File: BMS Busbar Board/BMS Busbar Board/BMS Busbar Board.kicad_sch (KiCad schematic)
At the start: 17 parts, among them J1 Conn_01x05_MountingPin, J2 Conn_01x05_MountingPin

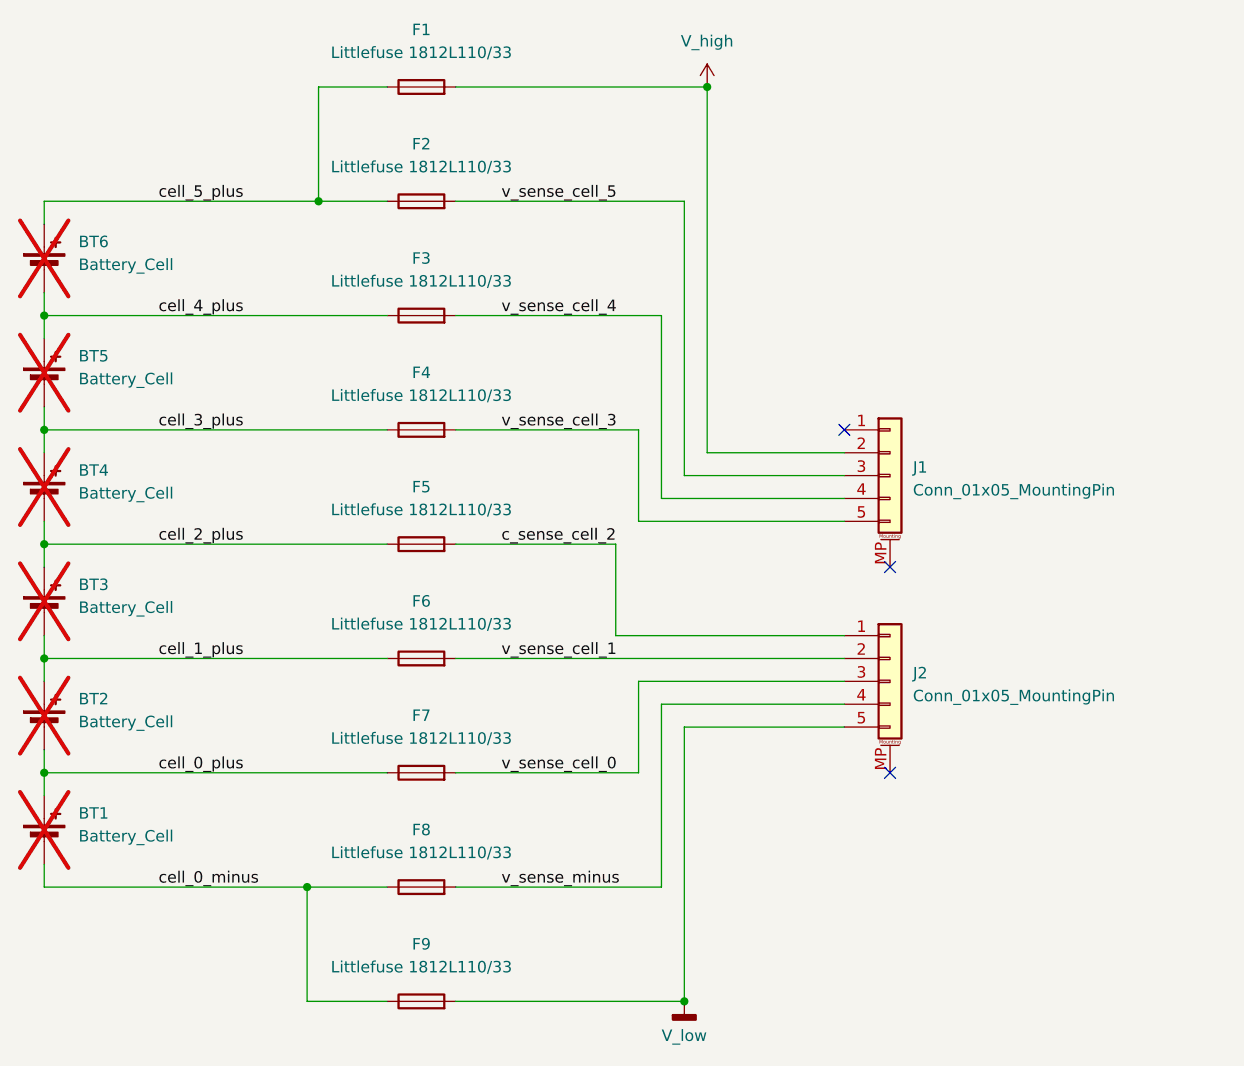
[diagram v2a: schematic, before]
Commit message: new connector added
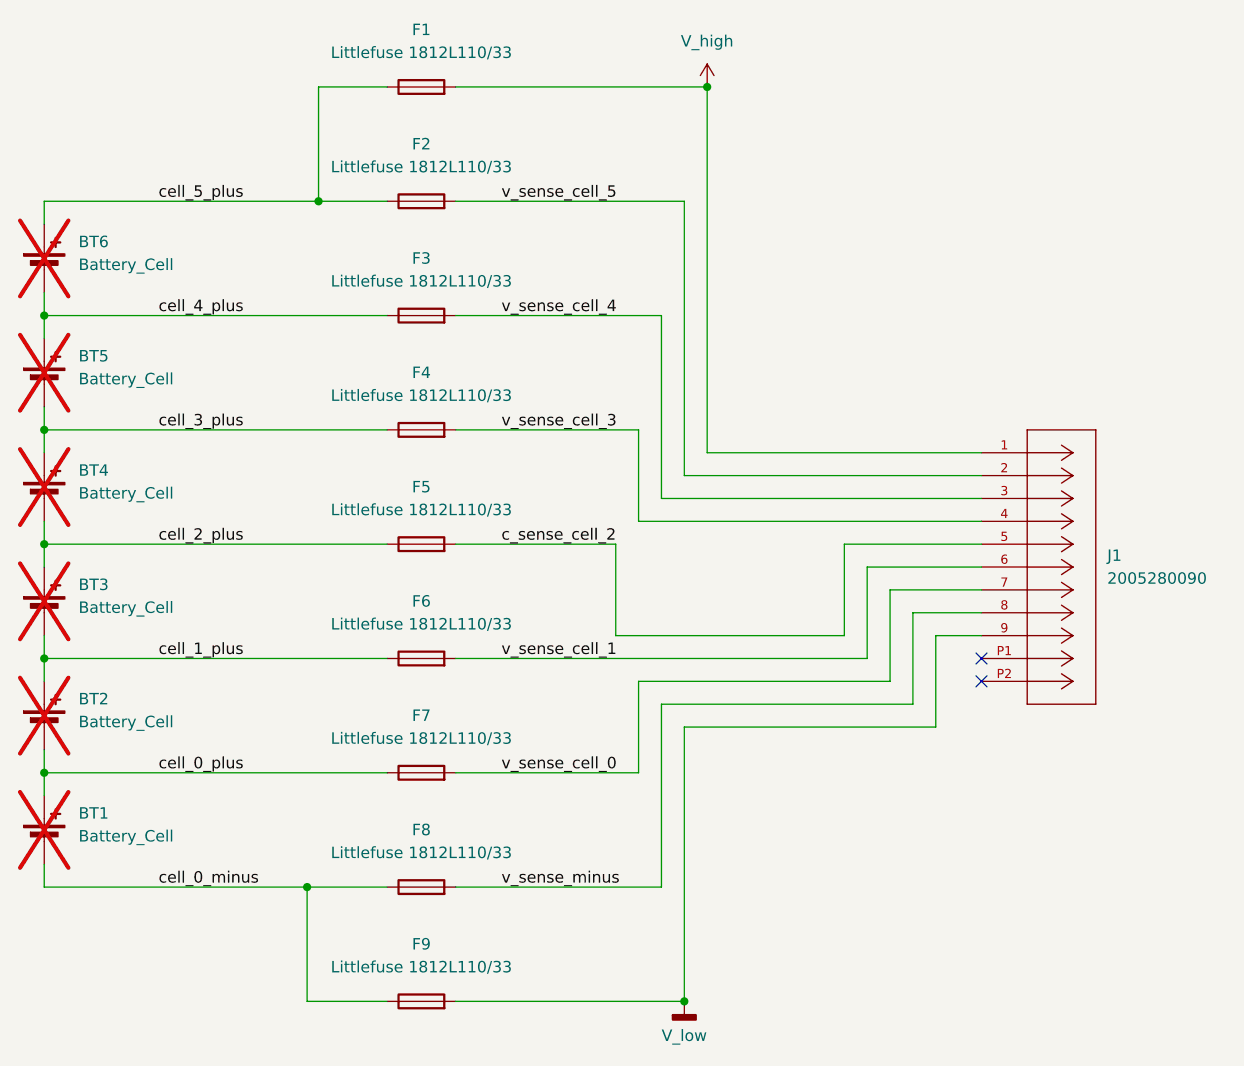
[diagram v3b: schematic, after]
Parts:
- removed J1, J2: Conn_01x05_MountingPin, FS_4_Global_Footprint_Library:512810598, symbol Connector_Generic_MountingPin:Conn_01x05_MountingPin
- added J1: 2005280090, FS_4_Global_Footprint_Library:CON_2005280090_MOL, symbol FS_4_Global_Symbol_Library:2005280090
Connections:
- net V_high: now also J1.1
- net V_low: now also J1.9
- net c_sense_cell_2: now also J1.5
- net v_sense_cell_0: now also J1.7
- net v_sense_cell_1: now also J1.6
- net v_sense_cell_3: now also J1.4
- net v_sense_cell_4: now also J1.3
- net v_sense_cell_5: now also J1.2
- net v_sense_minus: now also J1.8
- no-connect marks 3 -> 2
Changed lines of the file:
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@@
 	)
 	(no_connect
-		(at 157.48 104.14)
+		(at 167.64 93.98)
 	)
 	(no_connect
-		(at 157.48 81.28)
-	)
-	(no_connect
-		(at 152.4 66.04)
-	)
-	(wire
-		(pts
-			(xy 137.16 68.58) (xy 152.4 68.58)
+		(at 167.64 91.44)
+	)
+	(wire
+		(pts
+			(xy 160.02 86.36) (xy 167.64 86.36)
+		)
+		(stroke
+			(width 0)
+			(type default)
+		)
+	)
+	(wire
+		(pts
+			(xy 137.16 68.58) (xy 167.64 68.58)
 		)
 		(stroke
@@
 	(wire
 		(pts
-			(xy 134.62 99.06) (xy 152.4 99.06)
+			(xy 134.62 99.06) (xy 162.56 99.06)
 		)
 		(stroke
@@
 	(wire
 		(pts
-			(xy 129.54 93.98) (xy 152.4 93.98)
+			(xy 129.54 93.98) (xy 157.48 93.98)
 		)
 		(stroke
@@
 	(wire
 		(pts
-			(xy 109.22 91.44) (xy 152.4 91.44)
+			(xy 109.22 91.44) (xy 154.94 91.44)
 		)
 		(stroke
@@
 	(wire
 		(pts
+			(xy 157.48 93.98) (xy 157.48 83.82)
+		)
+		(stroke
+			(width 0)
+			(type default)
+		)
+	)
+	(wire
+		(pts
 			(xy 101.6 91.44) (xy 63.5 91.44)
 		)
@@
 	(wire
 		(pts
+			(xy 162.56 99.06) (xy 162.56 88.9)
+		)
+		(stroke
+			(width 0)
+			(type default)
+		)
+	)
+	(wire
+		(pts
 			(xy 63.5 114.3) (xy 63.5 116.84)
 		)
@@
 	(wire
 		(pts
+			(xy 154.94 91.44) (xy 154.94 81.28)
+		)
+		(stroke
+			(width 0)
+			(type default)
+		)
+	)
+	(wire
+		(pts
 			(xy 63.5 88.9) (xy 63.5 91.44)
 		)
@@
 	(wire
 		(pts
+			(xy 152.4 88.9) (xy 152.4 78.74)
+		)
+		(stroke
+			(width 0)
+			(type default)
+		)
+	)
+	(wire
+		(pts
 			(xy 63.5 104.14) (xy 63.5 106.68)
 		)
@@
 	(wire
 		(pts
-			(xy 129.54 76.2) (xy 152.4 76.2)
+			(xy 162.56 88.9) (xy 167.64 88.9)
+		)
+		(stroke
+			(width 0)
+			(type default)
+		)
+	)
+	(wire
+		(pts
+			(xy 129.54 76.2) (xy 167.64 76.2)
 		)
 		(stroke
@@
 	(wire
 		(pts
+			(xy 160.02 96.52) (xy 160.02 86.36)
+		)
+		(stroke
+			(width 0)
+			(type default)
+		)
+	)
+	(wire
+		(pts
 			(xy 132.08 53.34) (xy 132.08 73.66)
 		)
@@
 	(wire
 		(pts
-			(xy 132.08 96.52) (xy 152.4 96.52)
-		)
-		(stroke
-			(width 0)
-			(type default)
-		)
-	)
-	(wire
-		(pts
-			(xy 132.08 73.66) (xy 152.4 73.66)
+			(xy 132.08 96.52) (xy 160.02 96.52)
+		)
+		(stroke
+			(width 0)
+			(type default)
+		)
+	)
+	(wire
+		(pts
+			(xy 132.08 73.66) (xy 167.64 73.66)
 		)
 		(stroke
@@
 	(wire
 		(pts
-			(xy 134.62 71.12) (xy 152.4 71.12)
+			(xy 134.62 71.12) (xy 167.64 71.12)
 		)
 		(stroke
@@
 	(wire
 		(pts
+			(xy 152.4 78.74) (xy 167.64 78.74)
+		)
+		(stroke
+			(width 0)
+			(type default)
+		)
+	)
+	(wire
+		(pts
+			(xy 154.94 81.28) (xy 167.64 81.28)
+		)
+		(stroke
+			(width 0)
+			(type default)
+		)
+	)
+	(wire
+		(pts
 			(xy 63.5 101.6) (xy 63.5 104.14)
 		)
@@
 		(pts
 			(xy 109.22 129.54) (xy 134.62 129.54)
+		)
+		(stroke
+			(width 0)
+			(type default)
+		)
+	)
+	(wire
+		(pts
+			(xy 157.48 83.82) (xy 167.64 83.82)
 		)
 		(stroke
@@
 	)
 	(symbol
-		(lib_id "Connector_Generic_MountingPin:Conn_01x05_MountingPin")
-		(at 157.48 93.98 0)
-		(unit 1)
-		(exclude_from_sim no)
-		(in_bom yes)
-		(on_board yes)
-		(dnp no)
-		(property "Reference" "J2"
-			(at 160.02 93.0655 0)
-			(effects
-				(font
-					(size 1.27 1.27)
-				)
-				(justify left)
-			)
-		)
-		(property "Value" "Conn_01x05_MountingPin"
-			(at 160.02 95.6055 0)
-			(effects
-				(font
-					(size 1.27 1.27)
-				)
-				(justify left)
-			)
-		)
-		(property "Footprint" "FS_4_Global_Footprint_Library:512810598"
-			(at 157.48 93.98 0)
-			(effects
-				(font
-					(size 1.27 1.27)
-				)
-				(hide yes)
-			)
-		)
-		(property "Datasheet" "~"
-			(at 157.48 93.98 0)
-			(effects
-				(font
-					(size 1.27 1.27)
-				)
-				(hide yes)
-			)
-		)
-		(property "Description" "Generic connectable mounting pin connector, single row, 01x05, script generated (kicad-library-utils/schlib/autogen/connector/)"
-			(at 157.48 93.98 0)
-			(effects
-				(font
-					(size 1.27 1.27)
-				)
-				(hide yes)
-			)
-		)
-		(pin "1"
-		)
-		(pin "5"
-		)
-		(pin "4"
-		)
-		(pin "3"
-		)
-		(pin "2"
-		)
-		(pin "MP"
-		)
-		(instances
-			(project "BMS Busbar Board"
-				(path "/4a7933dc-894e-4333-8e50-6627480f7b53"
-					(reference "J2")
-					(unit 1)
-				)
-			)
-		)
-	)
-	(symbol
 		(lib_id "Device:Fuse")
 		(at 105.41 129.54 90)
@@
 	)
 	(symbol
+		(lib_id "FS_4_Global_Symbol_Library:2005280090")
+		(at 167.64 68.58 0)
+		(unit 1)
+		(exclude_from_sim no)
+		(in_bom yes)
+		(on_board yes)
+		(dnp no)
+		(fields_autoplaced yes)
+		(property "Reference" "J1"
+			(at 181.61 80.0099 0)
+			(effects
+				(font
+					(size 1.27 1.27)
+				)
+				(justify left)
+			)
+		)
+		(property "Value" "2005280090"
+			(at 181.61 82.5499 0)
+			(effects
+				(font
+					(size 1.27 1.27)
+				)
+				(justify left)
+			)
+		)
+		(property "Footprint" "FS_4_Global_Footprint_Library:CON_2005280090_MOL"
+			(at 172.974 58.928 0)
+			(effects
+				(font
+					(size 1.27 1.27)
+				)
+				(justify bottom)
+				(hide yes)
+			)
+		)
+		(property "Datasheet" ""
+			(at 167.64 68.58 0)
+			(effects
+				(font
+					(size 1.27 1.27)
+				)
+				(hide yes)
+			)
+		)
+		(property "Description" ""
+			(at 167.64 68.58 0)
+			(effects
+				(font
+					(size 1.27 1.27)
+				)
+				(hide yes)
+			)
+		)
+		(pin "P2"
+		)
+		(pin "8"
+		)
+		(pin "P1"
+		)
+		(pin "2"
+		)
+		(pin "1"
+		)
+		(pin "5"
+		)
+		(pin "6"
+		)
+		(pin "3"
+		)
+		(pin "7"
+		)
+		(pin "9"
+		)
+		(pin "4"
+		)
+		(instances
+			(project ""
+				(path "/4a7933dc-894e-4333-8e50-6627480f7b53"
+					(reference "J1")
+					(unit 1)
+				)
+			)
+		)
+	)
+	(symbol
 		(lib_id "power:GNDD")
 		(at 134.62 129.54 0)
@@
 					(unit 1)
 				)
-			)
-		)
-	)
-	(symbol
-		(lib_id "Connector_Generic_MountingPin:Conn_01x05_MountingPin")
-		(at 157.48 71.12 0)
-		(unit 1)
-		(exclude_from_sim no)
-		(in_bom yes)
-		(on_board yes)
-		(dnp no)
-		(property "Reference" "J1"
-			(at 160.02 70.2055 0)
-			(effects
-				(font
-					(size 1.27 1.27)
-				)
-				(justify left)
-			)
-		)
-		(property "Value" "Conn_01x05_MountingPin"
-			(at 160.02 72.7455 0)
-			(effects
-				(font
-					(size 1.27 1.27)
-				)
-				(justify left)
-			)
-		)
-		(property "Footprint" "FS_4_Global_Footprint_Library:512810598"
-			(at 157.48 71.12 0)
-			(effects
-				(font
-					(size 1.27 1.27)
-				)
-				(hide yes)
-			)
-		)
-		(property "Datasheet" "~"
-			(at 157.48 71.12 0)
-			(effects
-				(font
-					(size 1.27 1.27)
-				)
-				(hide yes)
-			)
-		)
-		(property "Description" "Generic connectable mounting pin connector, single row, 01x05, script generated (kicad-library-utils/schlib/autogen/connector/)"
-			(at 157.48 71.12 0)
-			(effects
-				(font
-					(size 1.27 1.27)
-				)
-				(hide yes)
-			)
-		)
-		(pin "1"
-		)
-		(pin "5"
-		)
-		(pin "4"
-		)
-		(pin "3"
-		)
-		(pin "2"
-		)
-		(pin "MP"
-		)
-		(instances
-			(project ""
-				(path "/4a7933dc-894e-4333-8e50-6627480f7b53"
-					(reference "J1")
-					(unit 1)
-				)
